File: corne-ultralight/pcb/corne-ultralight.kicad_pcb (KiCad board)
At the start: 2 copper layers, 275.5 x 105.6 mm, 132 parts, among them J2 OLED, J5 Breakaway_Tabs, J7 OLED, SW1 SW_PUSH, SW10 SW_PUSH, SW11 SW_PUSH, SW12 SW_PUSH, SW13 SW_PUSH, SW14 SW_PUSH, SW15 SW_PUSH, SW16 SW_PUSH, SW17 SW_PUSH, SW18 SW_PUSH, SW19 SW_PUSH, SW2 SW_PUSH, SW20 SW_PUSH, SW21 SW_PUSH, SW22 SW_PUSH, SW23 SW_PUSH, SW24 SW_PUSH, SW25 SW_PUSH, SW26 SW_PUSH, SW27 SW_PUSH, SW28 SW_PUSH, SW29 SW_PUSH, SW3 SW_PUSH, SW30 SW_PUSH, SW31 SW_PUSH, SW32 SW_PUSH, SW33 SW_PUSH, SW34 SW_PUSH, SW35 SW_PUSH, SW36 SW_PUSH, SW37 SW_PUSH, SW38 SW_PUSH, SW39 SW_PUSH, SW4 SW_PUSH, SW40 SW_PUSH, SW41 SW_PUSH, SW42 SW_PUSH, SW5 SW_PUSH, SW6 SW_PUSH, SW7 SW_PUSH, SW8 SW_PUSH, SW9 SW_PUSH, U1 ProMicro, U2 ProMicro

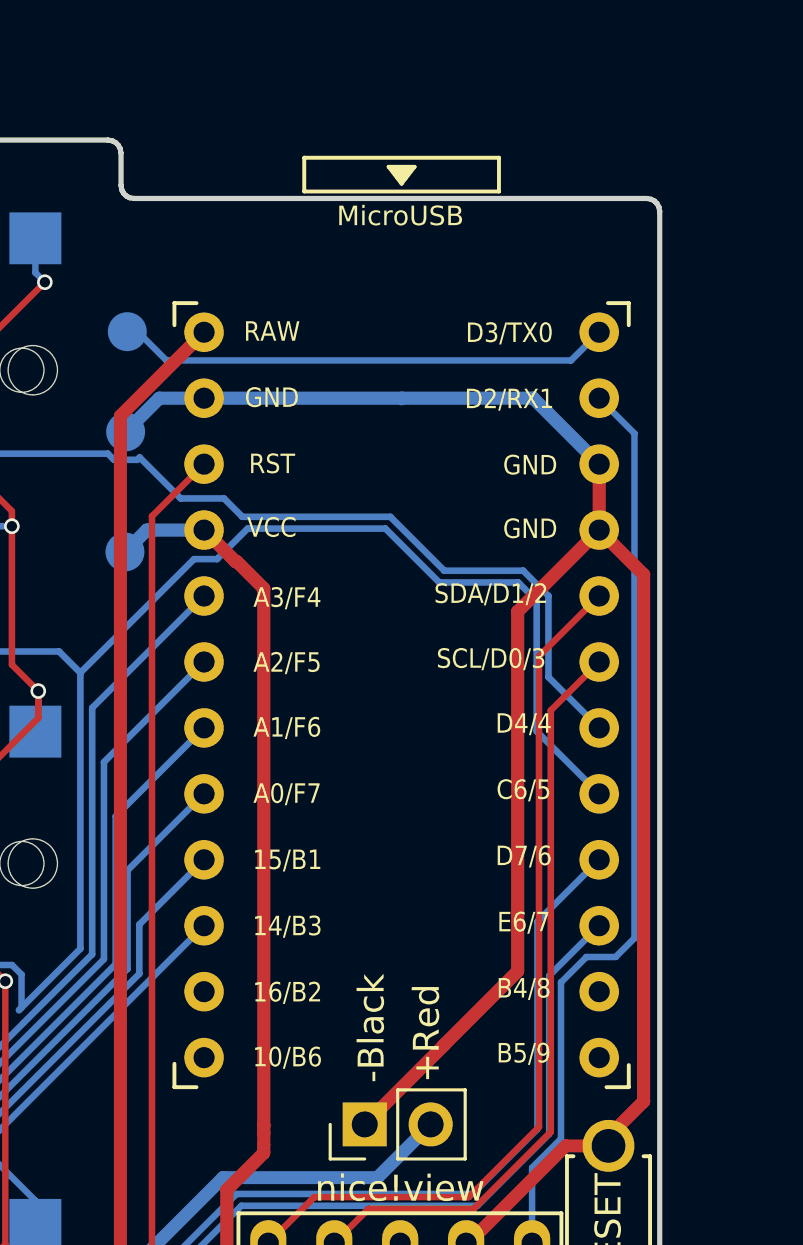
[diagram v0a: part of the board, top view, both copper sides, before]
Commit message: WIP
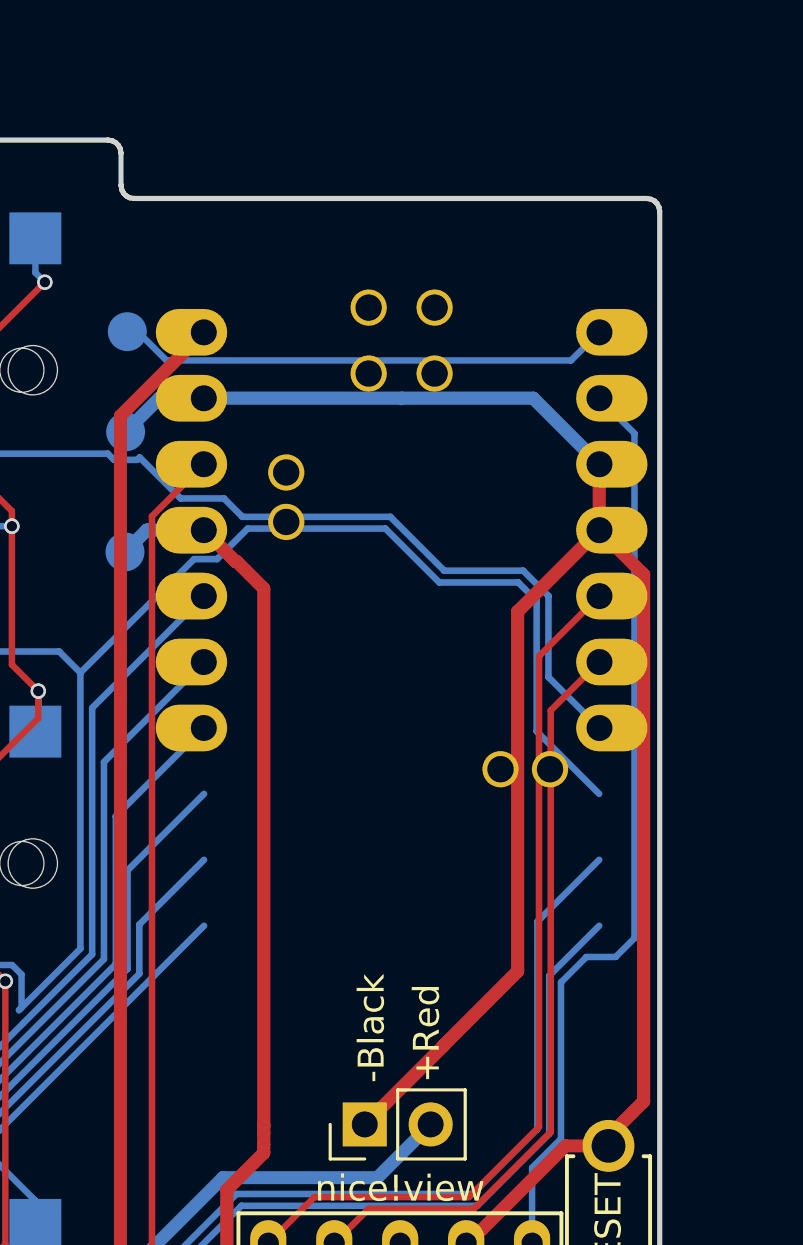
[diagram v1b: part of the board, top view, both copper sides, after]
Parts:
- U1: value ProMicro -> xiao-ble; footprint kbd:ProMicro_v3 -> kleeb-mcu:xiao-ble-tht
- moved U1 6.85 mm to (136.9, 49.7)
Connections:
- U1 pad 1: RGB -> row0
- U1 pad 10: row3 -> col3
- U1 pad 11: unconnected-(U1-Pad11) -> col2
- U1 pad 12: unconnected-(U1-Pad12) -> VCC
- U1 pad 13: unconnected-(U1-Pad13) -> GND
- U1 pad 14: unconnected-(U1-Pad14) -> +BATT
- U1 pad 15: col5 -> unconnected-(U1-Pad15)
- U1 pad 16: col4 -> unconnected-(U1-Pad16)
- U1 pad 17: col3 -> reset
- U1 pad 18: col2 -> +5V
- U1 pad 19: col1 -> unconnected-(U1-Pad19)
- U1 pad 2: CS -> row1
- U1 pad 20: col0 -> +5V
- U1 pad 21: VCC -> col0
- U1 pad 22: reset -> col1
- U1 pad 3: GND -> row2
- U1 pad 4: GND -> row3
- U1 pad 7: row0 -> CS
- U1 pad 8: row1 -> col5
- U1 pad 9: row2 -> col4
